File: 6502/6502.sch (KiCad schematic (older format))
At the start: 36 parts, among them J1 Jack-DC, SW1 SW_Push, U1 74LS08, U10 NHD-0420H1Z, U11 65C51N, U2 PAL24, U3 74LS154, U4 62256, U5 28C256, U6 65C02S, U7 62256, U8 65C22S, U9 65C22S, X1 ACO-4MHz, Y1 1.8432MHz

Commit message: Updates
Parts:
- removed C17: 0.1uF, Capacitor_THT:C_Disc_D3.4mm_W2.1mm_P2.50mm, symbol Device:C
- removed J1: Jack-DC, Connector_BarrelJack:BarrelJack_Horizontal, symbol Connector:Jack-DC
- removed unit 3 of U1
- removed U11: 65C51N, Package_DIP:DIP-28_W15.24mm_Socket, symbol 6502-rescue:65C51N-6502
- removed U4, U7: 62256, Package_DIP:DIP-28_W15.24mm_Socket, symbol 6502-rescue:62256-6502
- removed U5: 28C256, Socket:DIP_Socket-28_W11.9_W12.7_W15.24_W17.78_W18.5_3M_228-1277-00-0602J, symbol 6502-rescue:28C256-6502
- removed U6: 65C02S, Package_DIP:DIP-40_W15.24mm_Socket, symbol 6502-rescue:65C02S-6502
- removed U8, U9: 65C22S, Package_DIP:DIP-40_W15.24mm_Socket, symbol 6502-rescue:65C22S-6502
- added BT1: 3V, symbol Device:Battery_Cell
- added C16: 0.1uF, Capacitor_THT:C_Disc_D3.4mm_W2.1mm_P2.50mm, symbol Device:C
- added D2: 1N4733A, symbol Device:D
- added R4, R5, R6, R7: 1K, Resistor_THT:R_Axial_DIN0207_L6.3mm_D2.5mm_P7.62mm_Horizontal, symbol Device:R
- added SW2: SW_Push, Button_Switch_THT:SW_PUSH_6mm_H4.3mm, symbol Switch:SW_Push
- added unit 4 of U1
- added U11: 6551, Package_DIP:DIP-28_W15.24mm_Socket, symbol 6502Computer:6551
- added U12: 65C02S, symbol 6502Computer:65C02S
- added U4: AS6C4008-55PCN, Package_DIP:DIP-32_W15.24mm, symbol Memory_RAM:AS6C4008-55PCN
- added U5: 28C256, symbol Memory_EEPROM:28C256
- added U6: DS1511, symbol 6502Computer:DS1511
- added U7, U8: 6522, Package_DIP:DIP-40_W15.24mm_Socket, symbol 6502Computer:6522
- added U9: SN76489AN, symbol 6502Computer:SN76489AN
- R3: value 220 -> 220Ω
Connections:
- net labels added: AUDIO_OUT, BE, EXT_IN1, EXT_IN2, NMI, RAM_CS, RDY, RTC_CE, RTC_IRQ, RTC_PWR, RTC_SWQ, decode4, decode[0..4]
- net labels removed: RAM_CS1, RAM_CS2, decode[0..3]
- wire segments 269 -> 289
- no-connect marks 3 -> 2
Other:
- moved on the sheet: C15, U1A, U1B, U1E, U2

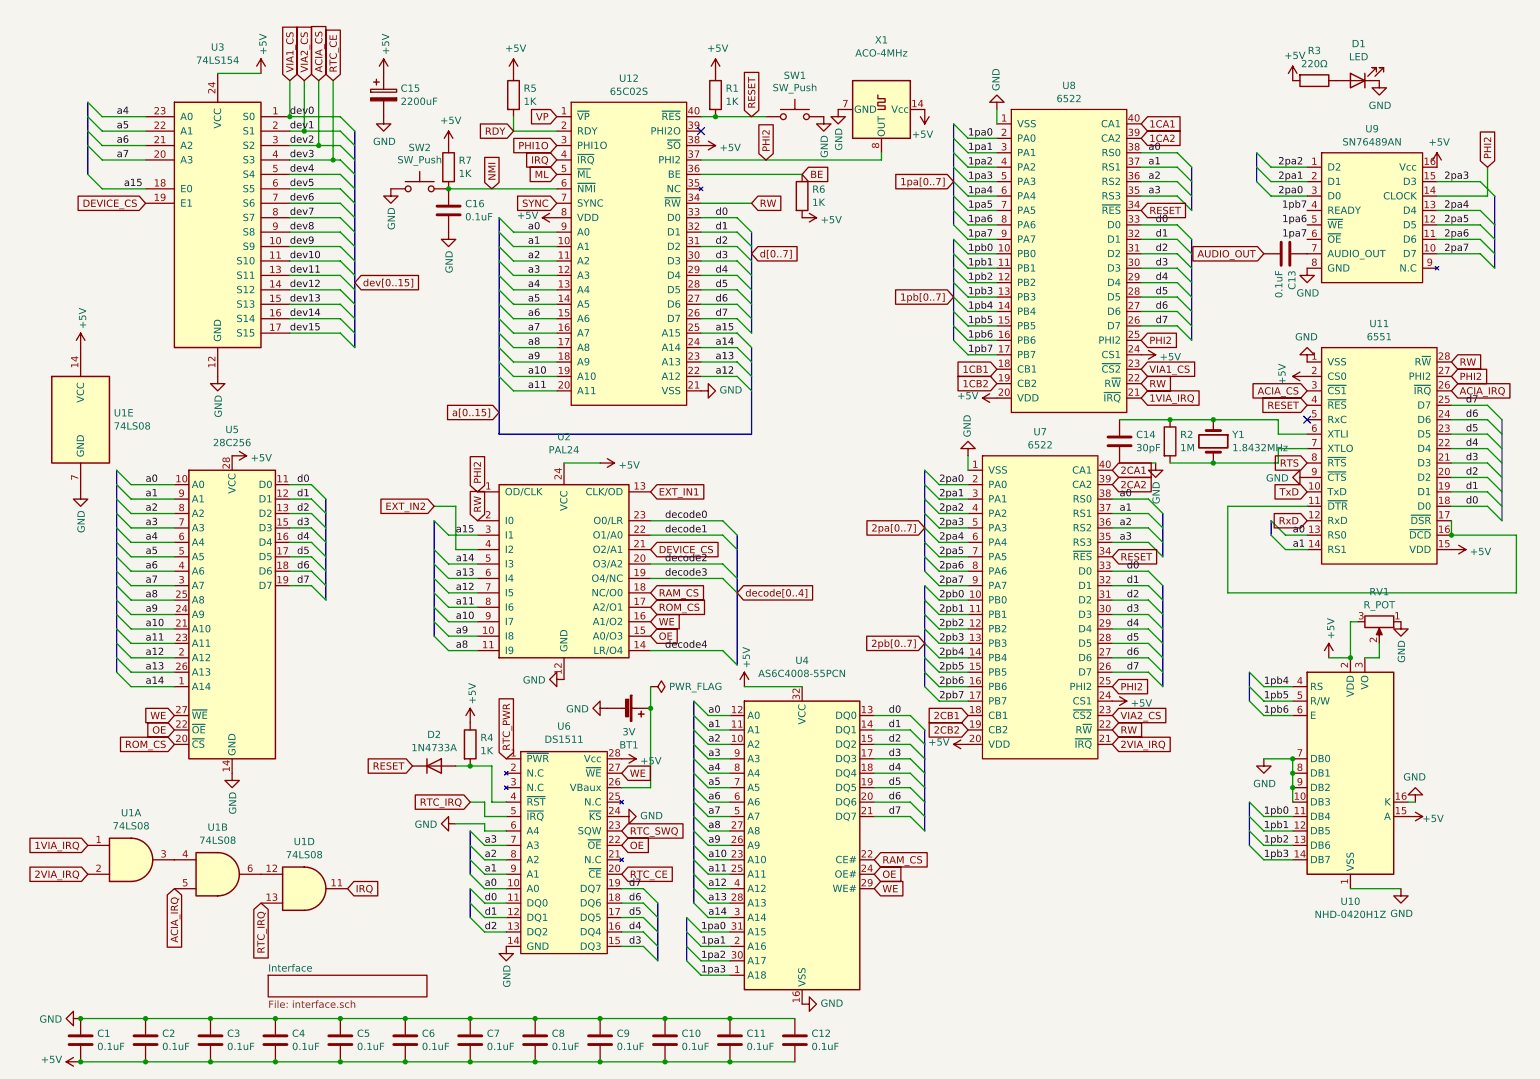
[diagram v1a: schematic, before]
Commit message: changes
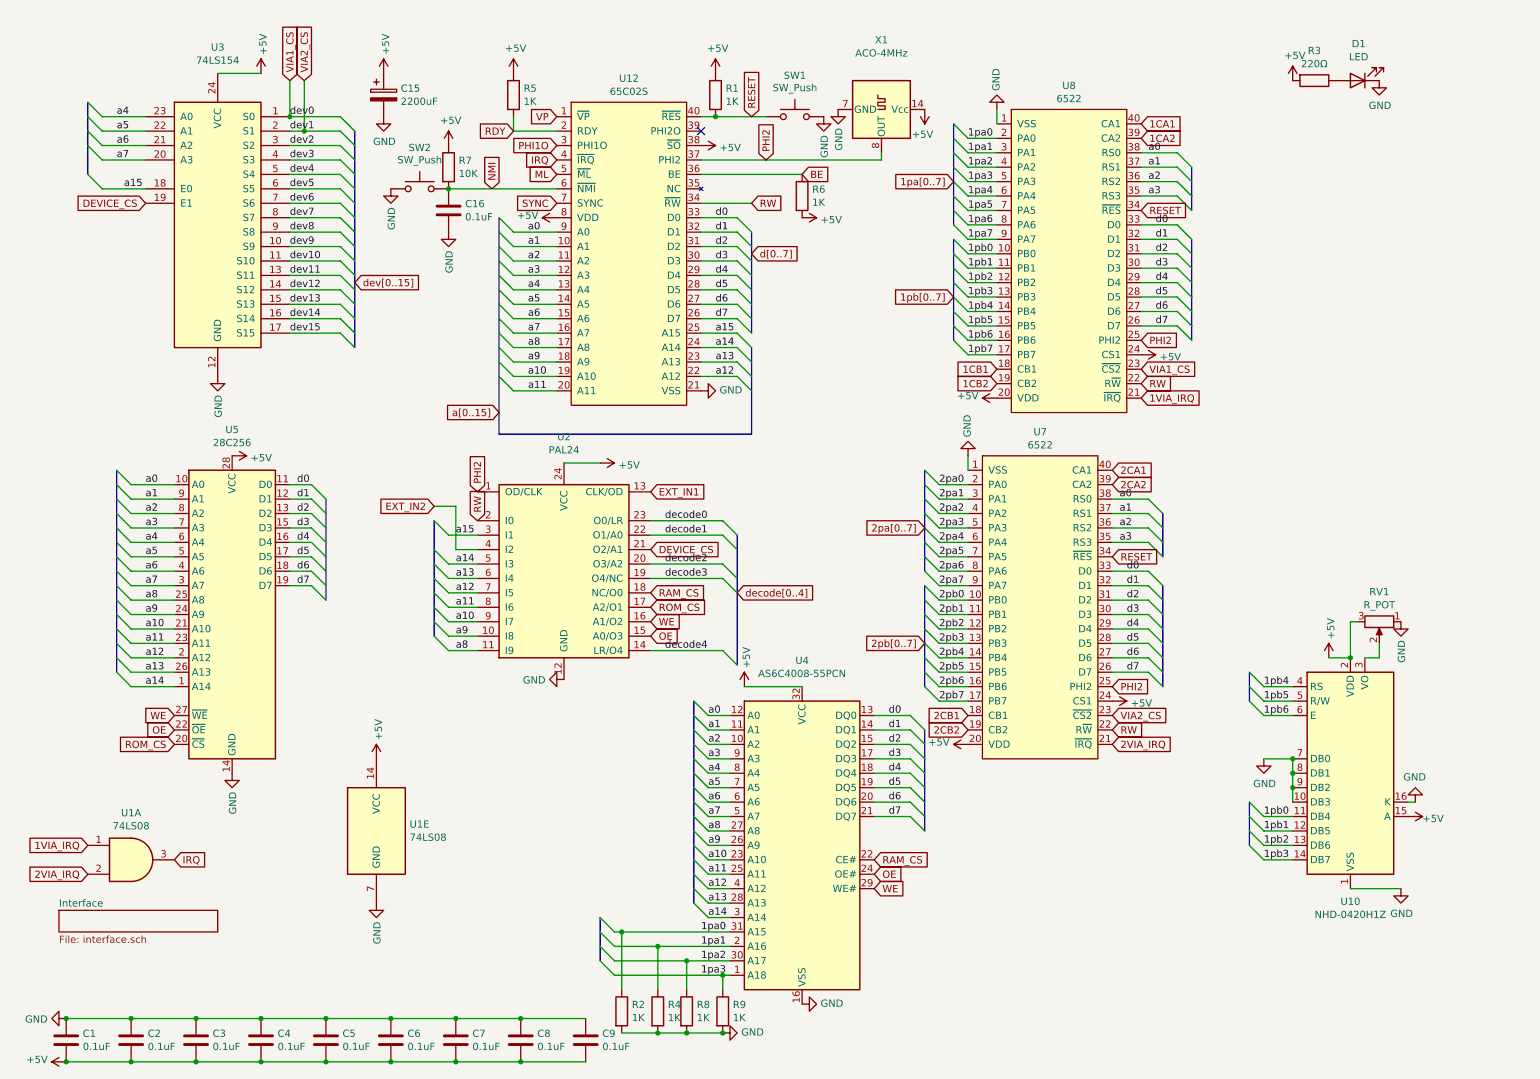
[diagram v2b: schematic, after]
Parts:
- removed BT1: 3V, symbol Device:Battery_Cell
- removed C10, C11, C12, C13: 0.1uF, Capacitor_THT:C_Disc_D3.4mm_W2.1mm_P2.50mm, symbol Device:C
- removed C14: 30pF, Capacitor_THT:C_Disc_D3.4mm_W2.1mm_P2.50mm, symbol Device:C
- removed D2: 1N4733A, symbol Device:D
- removed unit 2 of U1
- removed unit 4 of U1
- removed U11: 6551, Package_DIP:DIP-28_W15.24mm_Socket, symbol 6502Computer:6551
- removed U6: DS1511, symbol 6502Computer:DS1511
- removed U9: SN76489AN, symbol 6502Computer:SN76489AN
- removed Y1: 1.8432MHz, Crystal:Resonator-2Pin_W7.0mm_H2.5mm, symbol Device:Crystal
- added R8, R9: 1K, Resistor_THT:R_Axial_DIN0207_L6.3mm_D2.5mm_P7.62mm_Horizontal, symbol Device:R
- R2: value 1M -> 1K
- R7: value 1K -> 10K
- U10: footprint 6502:LCD-20x4 -> 6502Computer:LCD-20x4
- U12: footprint (none) -> Package_DIP:DIP-40_W15.24mm_Socket
- U4: footprint Package_DIP:DIP-32_W15.24mm -> Package_DIP:DIP-32_W15.24mm_Socket
- U5: footprint (none) -> 6502Computer:ZIF_Socket-28
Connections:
- net +5V: no longer R4.1
- net 1pa0: now also R2.1
- net 1pa1: now also R4.1
- net 1pa2: now also R8.1
- net 1pa3: now also R9.1
- net GND: now also R2.2, R4.2, R8.2, R9.2
- net IRQ: now also U1.3
- net ACIA_CS renamed dev2
- net RTC_CE renamed dev3
- no-connect marks 2 -> 1
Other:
- moved on the sheet: C1, C2, C3, C4, C5, C6, C7, C8, C9, U1E

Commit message: updates!
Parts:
- C1, C16, C2, C3, C4, C5, C6, C7, C8, C9: footprint Capacitor_THT:C_Disc_D3.4mm_W2.1mm_P2.50mm -> Capacitor_THT:C_Disc_D5.1mm_W3.2mm_P5.00mm
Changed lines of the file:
@@
 F 0 "C2" H 1315 7596 50  0000 L CNN
 F 1 "0.1uF" H 1315 7505 50  0000 L CNN
-F 2 "Capacitor_THT:C_Disc_D3.4mm_W2.1mm_P2.50mm" H 1238 7400 50  0001 C CNN
+F 2 "Capacitor_THT:C_Disc_D5.1mm_W3.2mm_P5.00mm" H 1238 7400 50  0001 C CNN
 F 3 "~" H 1200 7550 50  0001 C CNN
 	1    1200 7550
@@
 F 0 "C3" H 1765 7596 50  0000 L CNN
 F 1 "0.1uF" H 1765 7505 50  0000 L CNN
-F 2 "Capacitor_THT:C_Disc_D3.4mm_W2.1mm_P2.50mm" H 1688 7400 50  0001 C CNN
+F 2 "Capacitor_THT:C_Disc_D5.1mm_W3.2mm_P5.00mm" H 1688 7400 50  0001 C CNN
 F 3 "~" H 1650 7550 50  0001 C CNN
 	1    1650 7550
@@
 F 0 "C4" H 2215 7596 50  0000 L CNN
 F 1 "0.1uF" H 2215 7505 50  0000 L CNN
-F 2 "Capacitor_THT:C_Disc_D3.4mm_W2.1mm_P2.50mm" H 2138 7400 50  0001 C CNN
+F 2 "Capacitor_THT:C_Disc_D5.1mm_W3.2mm_P5.00mm" H 2138 7400 50  0001 C CNN
 F 3 "~" H 2100 7550 50  0001 C CNN
 	1    2100 7550
@@
 F 0 "C5" H 2665 7596 50  0000 L CNN
 F 1 "0.1uF" H 2665 7505 50  0000 L CNN
-F 2 "Capacitor_THT:C_Disc_D3.4mm_W2.1mm_P2.50mm" H 2588 7400 50  0001 C CNN
+F 2 "Capacitor_THT:C_Disc_D5.1mm_W3.2mm_P5.00mm" H 2588 7400 50  0001 C CNN
 F 3 "~" H 2550 7550 50  0001 C CNN
 	1    2550 7550
@@
 F 0 "C6" H 3115 7596 50  0000 L CNN
 F 1 "0.1uF" H 3115 7505 50  0000 L CNN
-F 2 "Capacitor_THT:C_Disc_D3.4mm_W2.1mm_P2.50mm" H 3038 7400 50  0001 C CNN
+F 2 "Capacitor_THT:C_Disc_D5.1mm_W3.2mm_P5.00mm" H 3038 7400 50  0001 C CNN
 F 3 "~" H 3000 7550 50  0001 C CNN
 	1    3000 7550
@@
 F 0 "C7" H 3565 7596 50  0000 L CNN
 F 1 "0.1uF" H 3565 7505 50  0000 L CNN
-F 2 "Capacitor_THT:C_Disc_D3.4mm_W2.1mm_P2.50mm" H 3488 7400 50  0001 C CNN
+F 2 "Capacitor_THT:C_Disc_D5.1mm_W3.2mm_P5.00mm" H 3488 7400 50  0001 C CNN
 F 3 "~" H 3450 7550 50  0001 C CNN
 	1    3450 7550
@@
 F 0 "C8" H 4015 7596 50  0000 L CNN
 F 1 "0.1uF" H 4015 7505 50  0000 L CNN
-F 2 "Capacitor_THT:C_Disc_D3.4mm_W2.1mm_P2.50mm" H 3938 7400 50  0001 C CNN
+F 2 "Capacitor_THT:C_Disc_D5.1mm_W3.2mm_P5.00mm" H 3938 7400 50  0001 C CNN
 F 3 "~" H 3900 7550 50  0001 C CNN
 	1    3900 7550
@@
 F 0 "C9" H 4465 7596 50  0000 L CNN
 F 1 "0.1uF" H 4465 7505 50  0000 L CNN
-F 2 "Capacitor_THT:C_Disc_D3.4mm_W2.1mm_P2.50mm" H 4388 7400 50  0001 C CNN
+F 2 "Capacitor_THT:C_Disc_D5.1mm_W3.2mm_P5.00mm" H 4388 7400 50  0001 C CNN
 F 3 "~" H 4350 7550 50  0001 C CNN
 	1    4350 7550
@@
 F 0 "C1" H 865 7596 50  0000 L CNN
 F 1 "0.1uF" H 865 7505 50  0000 L CNN
-F 2 "Capacitor_THT:C_Disc_D3.4mm_W2.1mm_P2.50mm" H 788 7400 50  0001 C CNN
+F 2 "Capacitor_THT:C_Disc_D5.1mm_W3.2mm_P5.00mm" H 788 7400 50  0001 C CNN
 F 3 "~" H 750 7550 50  0001 C CNN
 	1    750  7550
@@
 F 0 "C16" H 3515 1846 50  0000 L CNN
 F 1 "0.1uF" H 3515 1755 50  0000 L CNN
-F 2 "Capacitor_THT:C_Disc_D3.4mm_W2.1mm_P2.50mm" H 3438 1650 50  0001 C CNN
+F 2 "Capacitor_THT:C_Disc_D5.1mm_W3.2mm_P5.00mm" H 3438 1650 50  0001 C CNN
 F 3 "~" H 3400 1800 50  0001 C CNN
 	1    3400 1800
